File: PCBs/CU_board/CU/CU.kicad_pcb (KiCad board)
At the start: 2 copper layers, 83.8 x 137.2 mm, 48 parts, among them J1 Jack-DC, J10 Conn_01x04_Female, J11 Conn_01x04_Female, J12 Conn_01x04_Female, J13 Conn_01x15_Female, J14 Conn_01x15_Female, J2 Conn_01x04_Female, J3 Conn_01x04_Female, J4 Conn_01x04_Female, J5 Conn_01x04_Female, J6 Conn_01x04_Female, J7 Conn_01x08_Female, J8 Conn_01x04_Female, J9 Conn_01x08_Female, U1 LM317_3PinPackage

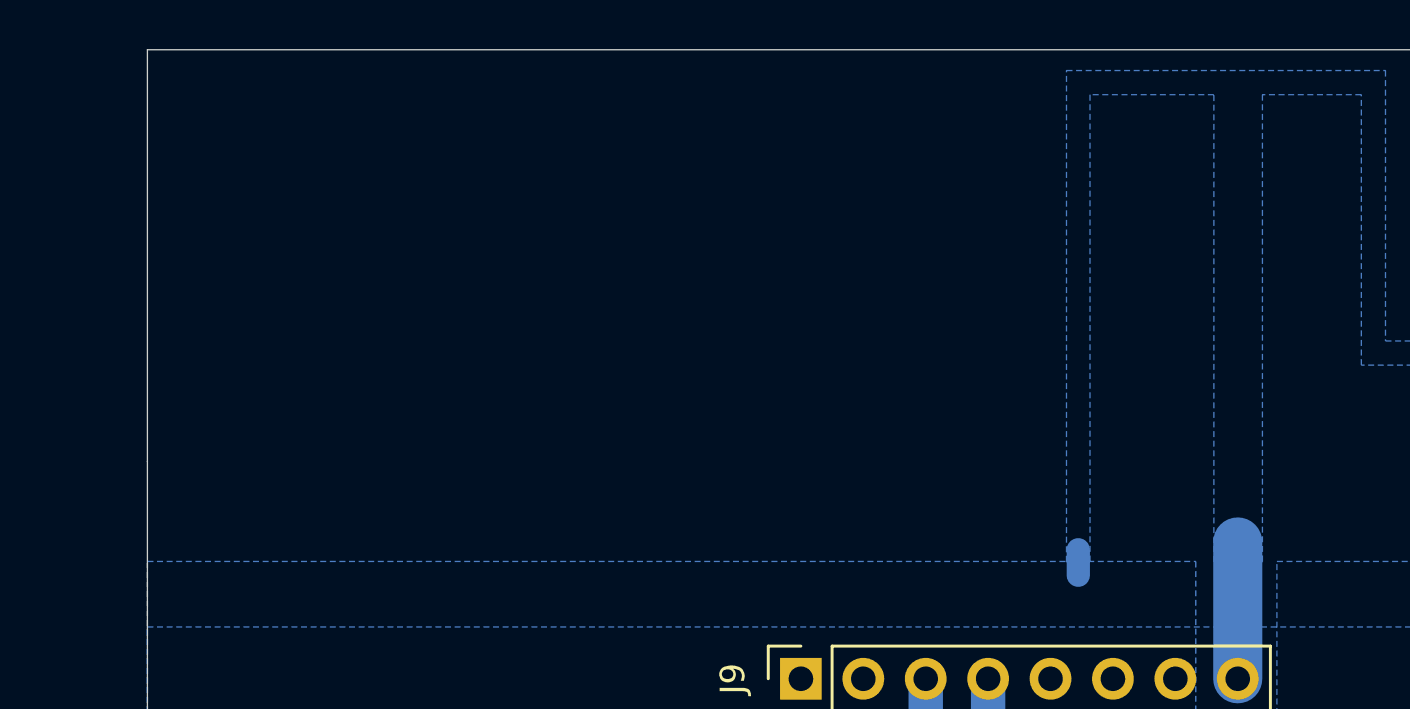
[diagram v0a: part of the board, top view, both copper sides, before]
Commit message: added gerbers
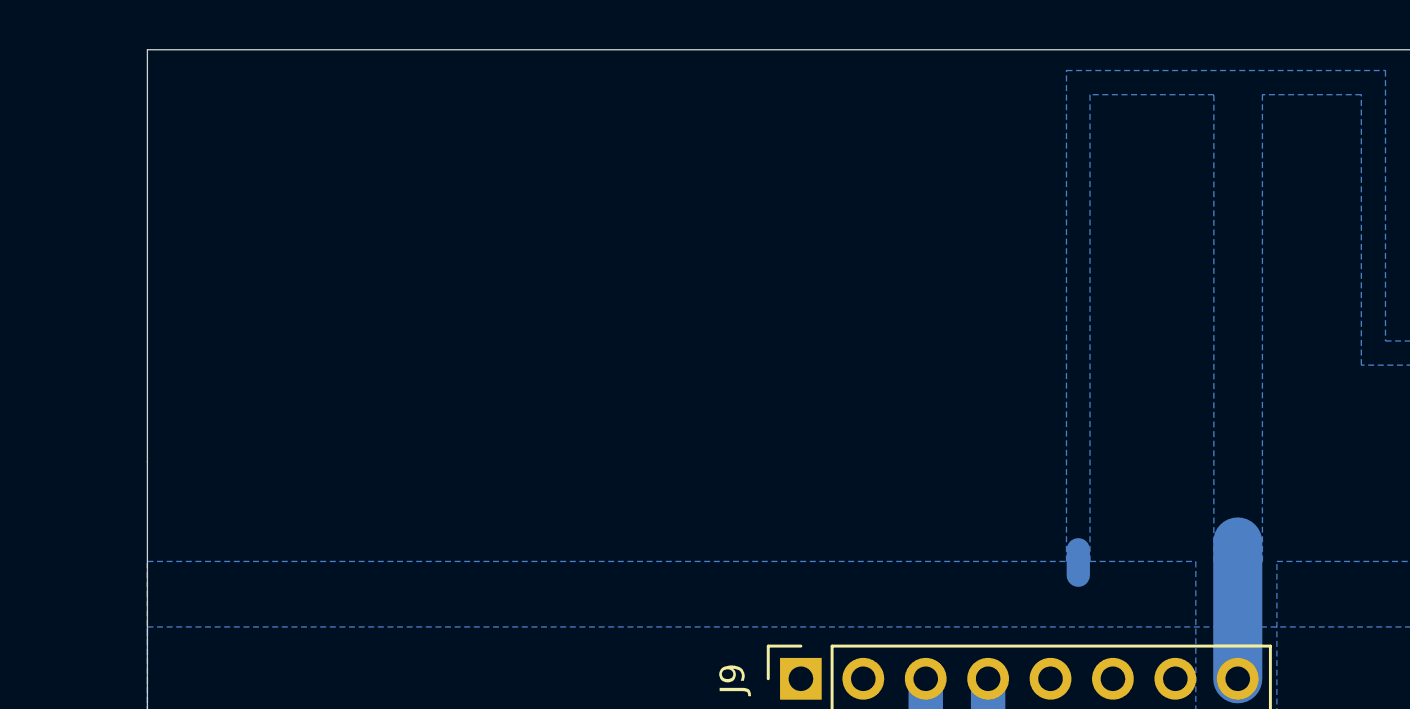
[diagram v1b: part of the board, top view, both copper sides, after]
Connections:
- J9 pad 8: Net-(J9-Pad8) -> Net-(J9-Pad7)
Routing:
- net Net-(J9-Pad7): track 0.00 -> 6.60 mm
- net Net-(J9-Pad8): track 5.57 -> 0.00 mm
- net (no net): track 1.04 -> 0.00 mm
- removed copper zone on B.Cu, net (none)
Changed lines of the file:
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@@
     (zones 0)
     (modules 48)
-    (nets 69)
+    (nets 68)
   )
   (page A4)
@@
   )
   (setup
-    (last_trace_width 0.95)
+    (last_trace_width 0.25)
     (user_trace_width 0.65)
     (user_trace_width 0.7)
@@
     (visible_elements 7FFFFFFF)
     (pcbplotparams
-      (layerselection 0x010fc_ffffffff)
+      (layerselection 0x01000_fffffffe)
       (usegerberextensions false)
       (usegerberattributes false)
@@
       (outputformat 1)
       (mirror false)
-      (drillshape 1)
+      (drillshape 0)
       (scaleselection 1)
       (outputdirectory ""))
@@
   (net 66 "Net-(R26-Pad1)")
   (net 67 "Net-(J10-Pad3)")
-  (net 68 "Net-(J9-Pad8)")
   (net_class Default "This is the default net class."
     (clearance 0.2)
@@
     (add_net "Net-(J9-Pad6)")
     (add_net "Net-(J9-Pad7)")
-    (add_net "Net-(J9-Pad8)")
     (add_net "Net-(R14-Pad2)")
     (add_net "Net-(R15-Pad1)")
@@
     (fp_line (start -1.27 -1.27) (end 0.635 -1.27) (layer F.Fab) (width 0.1))
     (pad 8 thru_hole oval (at 0 17.78 90) (size 1.7 1.7) (drill 1) (layers *.Cu *.Mask)
-      (net 68 "Net-(J9-Pad8)"))
+      (net 24 "Net-(J9-Pad7)"))
     (pad 7 thru_hole oval (at 0 15.24 90) (size 1.7 1.7) (drill 1) (layers *.Cu *.Mask)
       (net 24 "Net-(J9-Pad7)"))
@@
   (gr_line (start 142.24 44.704) (end 142.24 147.066) (layer Edge.Cuts) (width 0.05))
   (gr_line (start 58.42 88.646) (end 58.42 44.704) (layer Edge.Cuts) (width 0.05))
-  (segment (start 96.30918 48.29302) (end 96.30918 49.32934) (width 0.95) (layer B.Cu) (net 0))
   (segment (start 62.484 93.98) (end 64.516 93.98) (width 1.4) (layer B.Cu) (net 2))
   (segment (start 60.325 91.821) (end 62.484 93.98) (width 1.4) (layer B.Cu) (net 2))
@@
   (segment (start 133.223 150.495) (end 133.223 147.828) (width 1.4) (layer B.Cu) (net 23))
   (segment (start 127.635 156.083) (end 133.223 150.495) (width 1.4) (layer B.Cu) (net 23))
-  (segment (start 102.799873 53.542947) (end 102.799873 47.974527) (width 2) (layer B.Cu) (net 68))
   (segment (start 64.093779 67.429427) (end 63.553778 66.889426) (width 1) (layer B.Cu) (net 27))
   (segment (start 63.553778 66.889426) (end 61.553779 66.889428) (width 1) (layer B.Cu) (net 27))
@@
   (segment (start 83.592346 101.540868) (end 77.724 107.409214) (width 1.4) (layer B.Cu) (net 67))
   (segment (start 83.592346 100.338787) (end 83.592346 101.540868) (width 1.4) (layer B.Cu) (net 67))
-  (zone (net 0) (net_name "") (layer B.Cu) (hatch edge 0.508)
+  (segment (start 102.799873 53.542947) (end 102.799873 47.974527) (width 2) (layer B.Cu) (net 24))
+  (segment (start 96.30918 48.29302) (end 96.30918 49.32934) (width 0.95) (layer B.Cu) (net 24))
+  (zone (net 24) (net_name "Net-(J9-Pad7)") (layer B.Cu) (hatch edge 0.508)
+    (priority 5)
     (connect_pads (clearance 0.7))
     (min_thickness 0.65)
@@
         (xy 133.8326 40.77716) (xy 127.84074 40.77716) (xy 127.84074 29.7688) (xy 123.81484 29.7688) (xy 123.81484 40.77716)
         (xy 117.84838 40.77716) (xy 117.85346 29.7688) (xy 113.82248 29.7688) (xy 113.82248 40.77716) (xy 107.83062 40.77716)
-        (xy 107.83062 29.7688) (xy 103.80472 29.7688) (xy 103.80472 48.78578) (xy 103.80218 48.78578) (xy 101.8286 48.78578)
-        (xy 101.8286 29.7688) (xy 96.7867 29.7688) (xy 96.7867 48.78578) (xy 95.82912 48.78578) (xy 95.82912 28.78582)
-        (xy 108.8136 28.78582) (xy 108.8136 39.79418) (xy 112.8395 39.79418) (xy 112.8395 28.78582) (xy 118.81866 28.78582)
-        (xy 118.82628 39.79672) (xy 122.83186 39.79418) (xy 122.83186 28.78582) (xy 128.82372 28.78582) (xy 128.82372 39.79418)
-        (xy 132.84962 39.79164) (xy 132.842 28.78074)
+        (xy 107.83062 29.7688) (xy 103.80472 29.7688) (xy 103.80472 48.78578) (xy 101.8286 48.78578) (xy 101.8286 29.7688)
+        (xy 96.7867 29.7688) (xy 96.7867 48.768) (xy 101.092 48.768) (xy 101.092 55.372) (xy 104.394 55.372)
+        (xy 104.394 48.768) (xy 142.2908 48.768) (xy 142.24 165.1) (xy 58.42 165.1) (xy 58.42 48.768)
+        (xy 95.82912 48.768) (xy 95.82912 28.78582) (xy 108.8136 28.78582) (xy 108.8136 39.79418) (xy 112.8395 39.79418)
+        (xy 112.8395 28.78582) (xy 118.81866 28.78582) (xy 118.82628 39.79672) (xy 122.83186 39.79418) (xy 122.83186 28.78582)
+        (xy 128.82372 28.78582) (xy 128.82372 39.79418) (xy 132.84962 39.79164) (xy 132.842 28.78074)
       )
     )
-  )
-  (zone (net 24) (net_name "Net-(J9-Pad7)") (layer B.Cu) (hatch edge 0.508)
-    (priority 5)
-    (connect_pads (clearance 0.7))
-    (min_thickness 0.65)
-    (fill yes (arc_segments 32) (thermal_gap 0.65) (thermal_bridge_width 0.7))
-    (polygon
-      (pts
-        (xy 101.092 55.372) (xy 104.394 55.372) (xy 104.394 48.768) (xy 142.2908 48.768) (xy 142.24 165.1)
-        (xy 58.42 165.1) (xy 58.42 48.768) (xy 101.092 48.768)
-      )
-    )
